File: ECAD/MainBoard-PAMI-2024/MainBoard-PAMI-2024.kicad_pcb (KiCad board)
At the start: 2 copper layers, 79.5 x 96 mm, 119 parts, among them J1 Selecteur-Robot, J10 Serial, J11 Con_Batt, J12 BAU, J13 OLED, J2 USB_B, J3 Tirette, J4 Servo, J5 Sensor_Right, J6 Sensor_Left, J7 LeftMotor, J8 RightMotor, SW1 SW_SPDT, U1 ESP32-S3-WROOM-1, U2 AMS1117-3.3, U4 TMC2208_SILENTSTEPSTICK, U5 TMC2208_SILENTSTEPSTICK

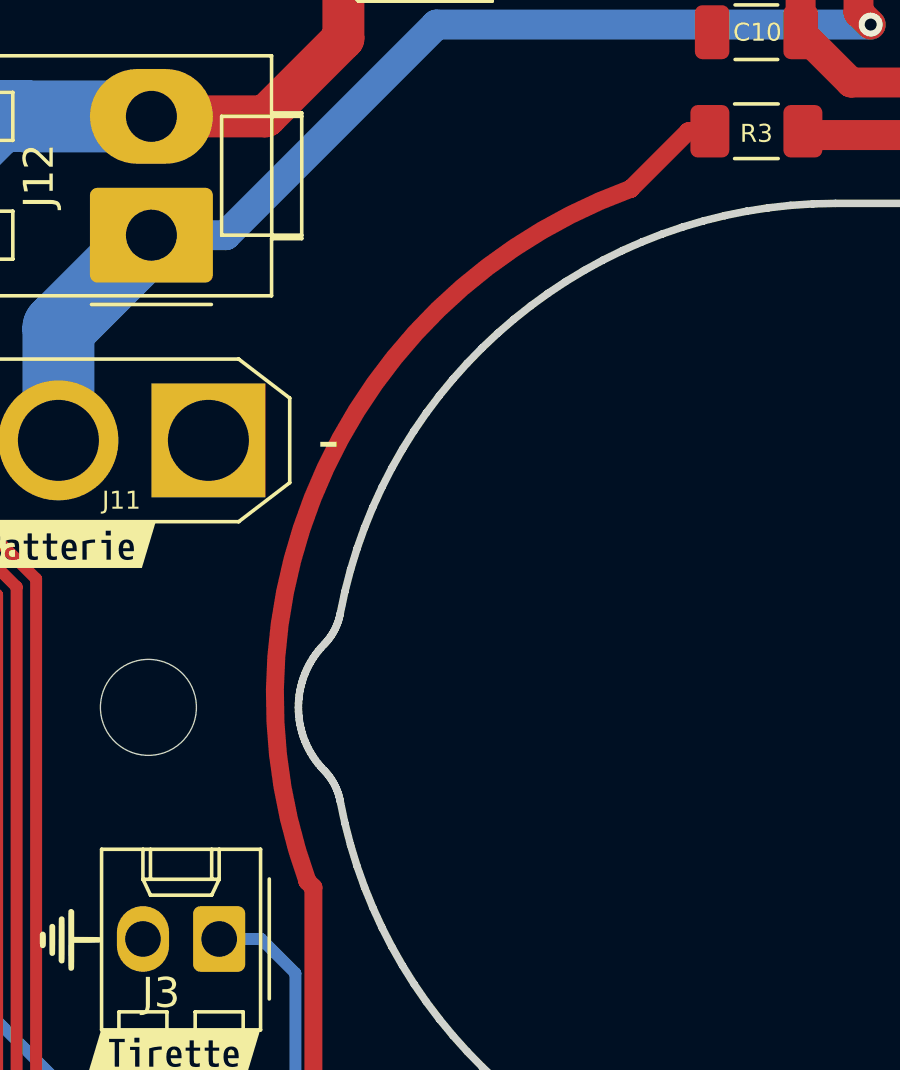
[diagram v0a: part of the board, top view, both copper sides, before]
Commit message: fix cutout
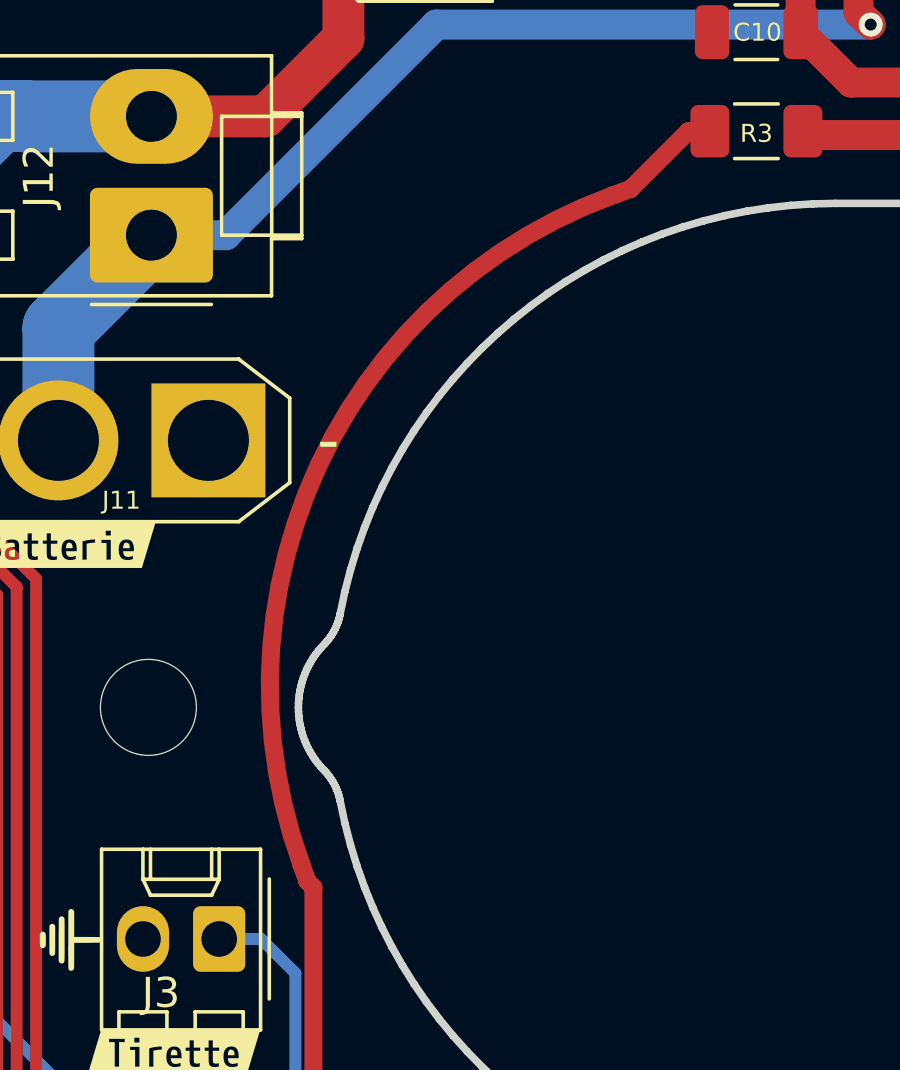
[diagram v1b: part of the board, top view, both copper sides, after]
